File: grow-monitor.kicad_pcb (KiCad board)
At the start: 4 copper layers, 20 x 140 mm, 62 parts, among them J1 PH 2.0, J2 I2C1, J3 DS18B20, M1 M5StampS3, M2 AHT21B, Q1 AO3401A, Q2 ALS-PT19-315C, Q3 AO3401A, Q4 2N7002, SW1 PWR2, SW2 CALIB, SW3 EN, SW4 PROG, SW5 KILL, SW6 PWR1, U1 SPX3819M5-L-3-3, U2 TPL5110, U5 NE555P

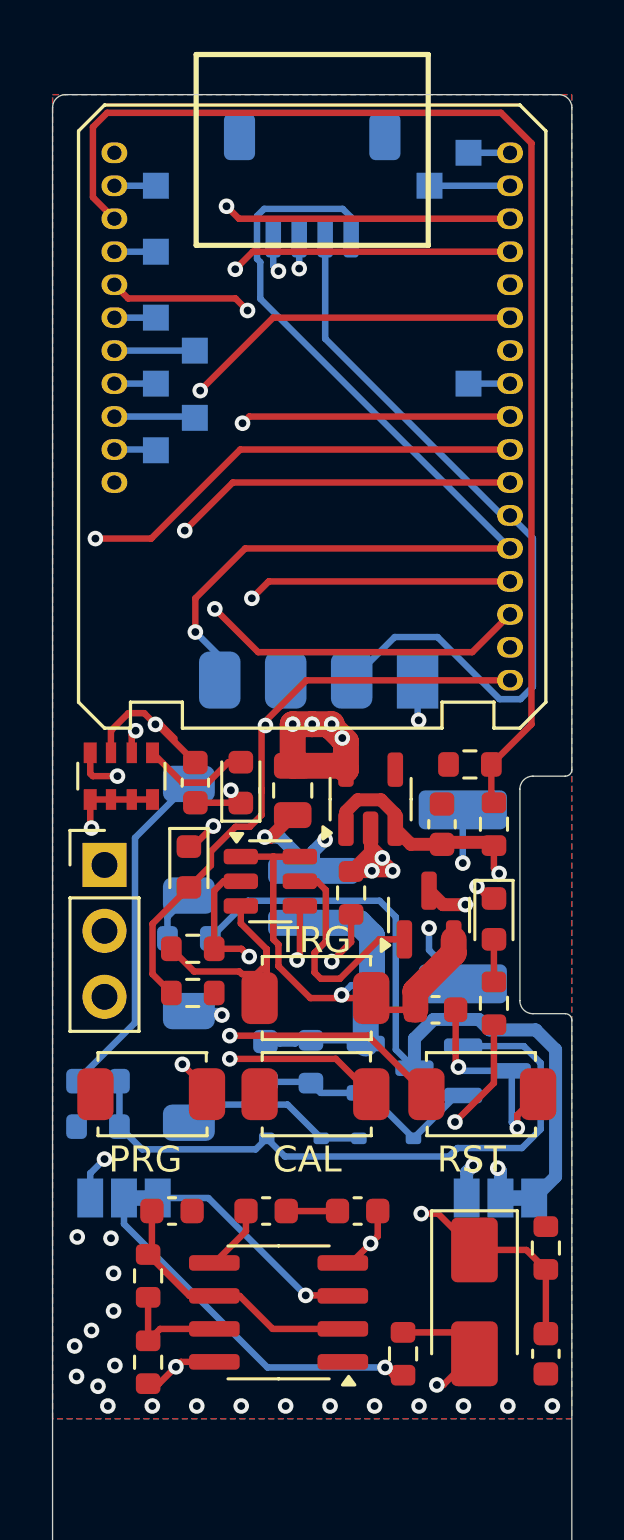
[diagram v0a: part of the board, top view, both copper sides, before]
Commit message: More tweaks
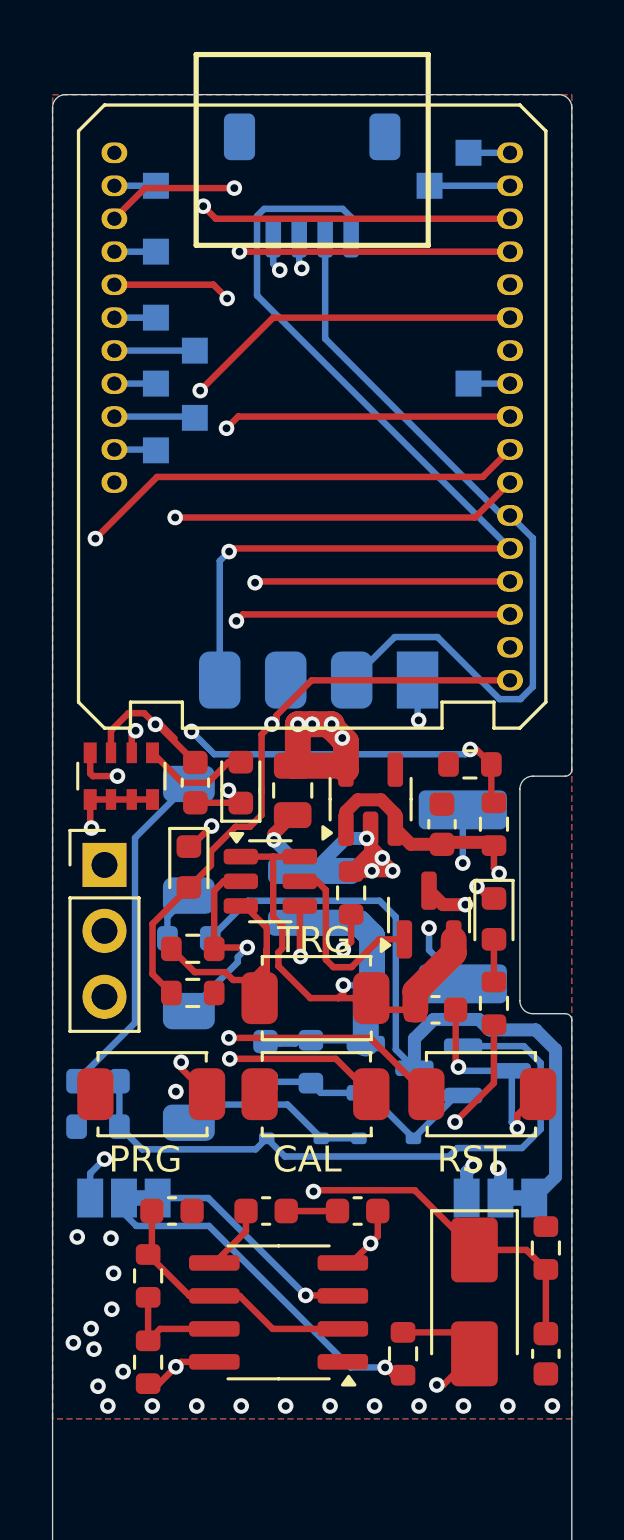
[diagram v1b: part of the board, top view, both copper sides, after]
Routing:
- net /TH_PWR: track 164.4 -> 157.5 mm, vias 3 -> 4
- net /B_VOLT: track 47.6 -> 41.6 mm, vias 0 -> 3
- net /S_SENSE: track 50.9 -> 47.9 mm
- net GND: track 128.4 -> 130.9 mm
- net Net-(Q1-G): track 8.68 -> 7.41 mm
- net /T_SENSE: track 164.1 -> 165.0 mm
- net /EN: track 52.0 -> 51.2 mm
- net Net-(D3-A): track 49.6 -> 49.8 mm, vias 2 -> 1
